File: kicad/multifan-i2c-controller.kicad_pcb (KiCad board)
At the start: 2 copper layers, 66 x 91.4 mm, 46 parts, among them J1 I2C, J2 Conn_01x02, J4 AVR-ISP-6, M1 Fan_Tacho_PWM, M2 Fan_Tacho_PWM, M3 Fan_Tacho_PWM, M4 Fan_Tacho_PWM, Q1 2N7000, Q2 2N7000, Q3 2N7000, Q4 2N7000, Q5 2N7000, Q6 2N7000, Q7 2N7000, Q8 2N7000, SW1 SW_Push, U1 ATmega328-P, Y1 16M

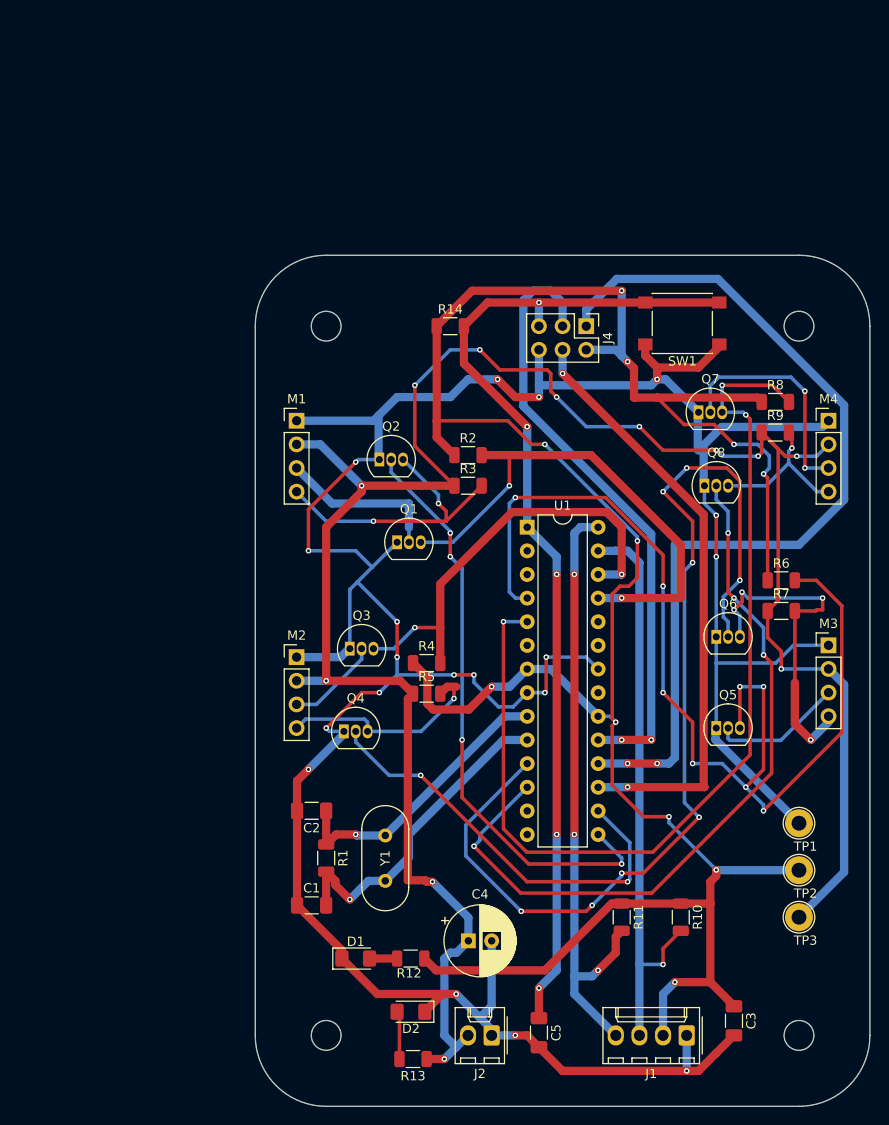
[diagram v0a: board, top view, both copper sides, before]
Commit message: revA
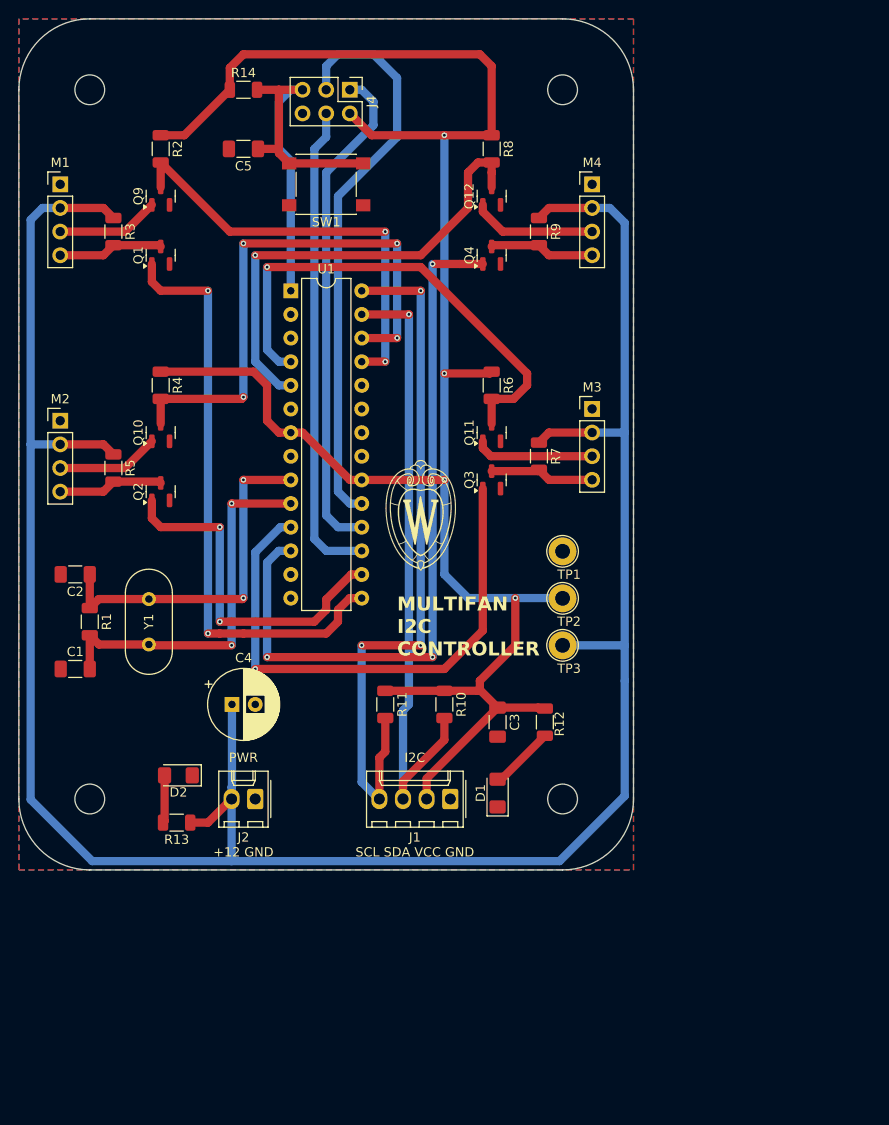
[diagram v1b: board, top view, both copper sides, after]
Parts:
- removed Q5, Q6, Q7, Q8: 2N7000, Package_TO_SOT_THT:TO-92_Inline
- removed the REF** at (101.6, 152.4)
- removed the REF** at (101.6, 76.2)
- removed the REF** at (152.4, 76.2)
- removed the REF** at (152.4, 152.4)
- added G***: LOGO, footprints:logo, F.Cu at (111.8, 96.5)
- added Q10: 2N7002, Package_TO_SOT_SMD:SOT-23, F.Cu at (83.8, 87.6)
- added Q11: 2N7002, Package_TO_SOT_SMD:SOT-23, F.Cu at (119.4, 87.6)
- added Q12: 2N7002, Package_TO_SOT_SMD:SOT-23, F.Cu at (119.4, 62.2)
- added Q9: 2N7002, Package_TO_SOT_SMD:SOT-23, F.Cu at (83.8, 62.2)
- added REF**: MountingHole_3.2mm_M3, MountingHole:MountingHole_3.2mm_M3, F.Cu at (76.2, 127.0)
- added REF**: MountingHole_3.2mm_M3, MountingHole:MountingHole_3.2mm_M3, F.Cu at (76.2, 50.8)
- added REF**: MountingHole_3.2mm_M3, MountingHole:MountingHole_3.2mm_M3, F.Cu at (127.0, 127.0)
- added REF**: MountingHole_3.2mm_M3, MountingHole:MountingHole_3.2mm_M3, F.Cu at (127.0, 50.8)
- added REF**: OSHW-Logo2_14.6x12mm_SilkScreen, Symbol:OSHW-Logo2_14.6x12mm_SilkScreen, B.Cu at (89.5, 77.5)
- Q1, Q2, Q3, Q4: value 2N7000 -> 2N7002; footprint Package_TO_SOT_THT:TO-92_Inline -> Package_TO_SOT_SMD:SOT-23
- moved C5 100.1 mm to (92.7, 57.1), turned to 180 degrees
- moved Q4 53.6 mm to (119.4, 68.6), turned to 90 degrees
- moved R3 46.9 mm to (78.7, 66.0), turned to -90 degrees
- moved R2 46.6 mm to (83.8, 57.1), turned to -90 degrees
- moved R5 41.5 mm to (78.7, 91.4), turned to -90 degrees
- moved R4 41.3 mm to (83.8, 82.5), turned to -90 degrees
- moved SW1 41.1 mm to (101.6, 61.0)
- moved C3 40.9 mm to (120.0, 118.7)
- moved R8 40.8 mm to (119.4, 57.1), turned to -90 degrees
- moved Q1 40.0 mm to (83.8, 68.6), turned to 90 degrees
- moved TP2 38.7 mm to (127.0, 105.4)
- moved TP1 38.7 mm to (127.0, 100.4)
- moved TP3 38.7 mm to (127.0, 110.5)
- moved R6 37.5 mm to (119.4, 82.5), turned to -90 degrees
- moved J1 35.9 mm to (114.9, 127.0)
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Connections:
- Q1 pad 1: GND -> /fan/PWM
- Q1 pad 2: Net-(M1-Tacho) -> GND
- Q1 pad 3: /fan/TACHO -> Net-(M1-PWM)
- Q2 pad 1: GND -> /fan1/PWM
- Q2 pad 2: /fan/PWM -> GND
- Q2 pad 3: Net-(M1-PWM) -> Net-(M2-PWM)
- Q3 pad 1: GND -> /fan2/PWM
- Q3 pad 2: Net-(M2-Tacho) -> GND
- Q3 pad 3: /fan1/TACHO -> Net-(M3-PWM)
- Q4 pad 1: GND -> /fan3/PWM
- Q4 pad 2: /fan1/PWM -> GND
- Q4 pad 3: Net-(M2-PWM) -> Net-(M4-PWM)
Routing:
- net GND: track 332.8 -> 0.00 mm, vias 19 -> 0
- net RESET: track 110.3 -> 47.4 mm, vias 5 -> 0
- net /fan2/TACHO: track 115.1 -> 53.0 mm, vias 8 -> 1
- net /fan3/TACHO: track 106.9 -> 50.7 mm, vias 3 -> 1
- net VCC: track 264.8 -> 210.2 mm, vias 11 -> 4
- net /fan2/PWM: track 109.4 -> 58.9 mm, vias 8 -> 1
- net MISO: track 98.2 -> 54.0 mm, vias 2 -> 0
- net +12V: track 234.3 -> 261.5 mm, vias 12 -> 0
- net Net-(M3-PWM): track 36.6 -> 11.3 mm, vias 4 -> 0
- net Net-(M1-PWM): track 31.3 -> 11.3 mm, vias 2 -> 0
- net MOSI: track 64.7 -> 51.9 mm, vias 2 -> 0
- net Net-(M2-PWM): track 23.3 -> 11.3 mm, vias 1 -> 0
- net Net-(M4-Tacho): track 24.8 -> 13.4 mm, vias 2 -> 0
- net /fan1/TACHO: track 47.6 -> 58.6 mm, vias 2 -> 4
- net SCL: track 66.7 -> 77.1 mm
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- added copper zone on B.Cu, net GND
- added copper zone on F.Cu, net GND
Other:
- board text added: "+12 GND"
- board text added: "I2C"
- board text added: "MULTIFAN I2C CONTROLLER"
- board text added: "PWR"
- board text added: "SCL SDA VCC GND"
- board text added: "https://github.com/ uw-madison-chem-shops/ multifan-i2c-controller"
